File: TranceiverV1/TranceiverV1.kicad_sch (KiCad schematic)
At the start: 21 parts, among them J1 Conn_01x03_Socket, J3 Battery, J4 Conn_01x03_Pin, M1 Motor_Servo, SW1 SW_Push_Open, U1 NRF24L01_, U3 102010388, U4 LD1086DTTR

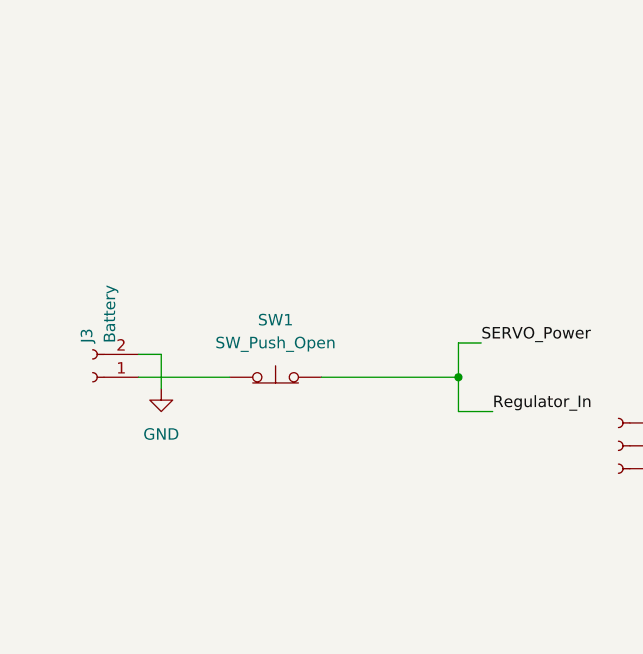
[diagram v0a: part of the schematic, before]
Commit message: changed switch
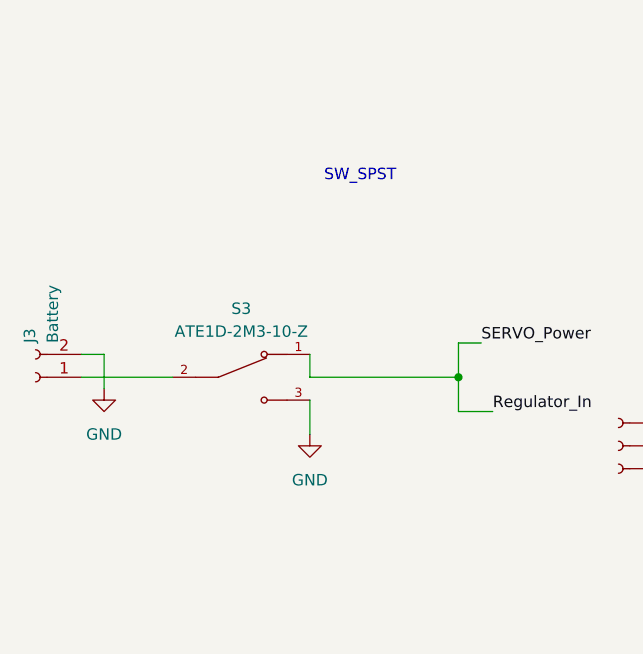
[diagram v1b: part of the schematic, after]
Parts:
- removed SW1: SW_Push_Open, Button_Switch_THT:SW_PUSH_1P1T_6x3.5mm_H5.0_APEM_MJTP1250, symbol Switch:SW_Push_Open
- added S3: ATE1D-2M3-10-Z, ATE1D-2M3-10-Z:SW_ATE1D-2M3-10-Z, symbol ATE1D-2M3-10-Z:ATE1D-2M3-10-Z
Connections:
- net GND: now also S3.3
- net Regulator_In: now also S3.1
- net at J3.1 (Pin_1): now also S3.2
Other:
- note added: "SW_SPST"
- moved on the sheet: J3
